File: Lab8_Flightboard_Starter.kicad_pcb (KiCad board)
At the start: 2 copper layers, 80 x 80 mm, 64 parts, among them J1 Motor1, J10 ESC3_GND, J11 ESC4_VBAT, J12 ESC4_GND, J2 Motor2, J3 Motor3, J4 Motor4, J5 ESC1_VBAT, J6 ESC1_GND, J7 ESC2_VBAT, J8 ESC2_GND, J9 ESC3_VBAT, Q1 DMP6023LE-13, U1 Teensy4.0, U2 TPS62933, U4 LP5912-3.3DRV, U5 LP5912-3.3DRV, U6 NRF24L01_Breakout, U9 LSM6DSO32_Adafruit

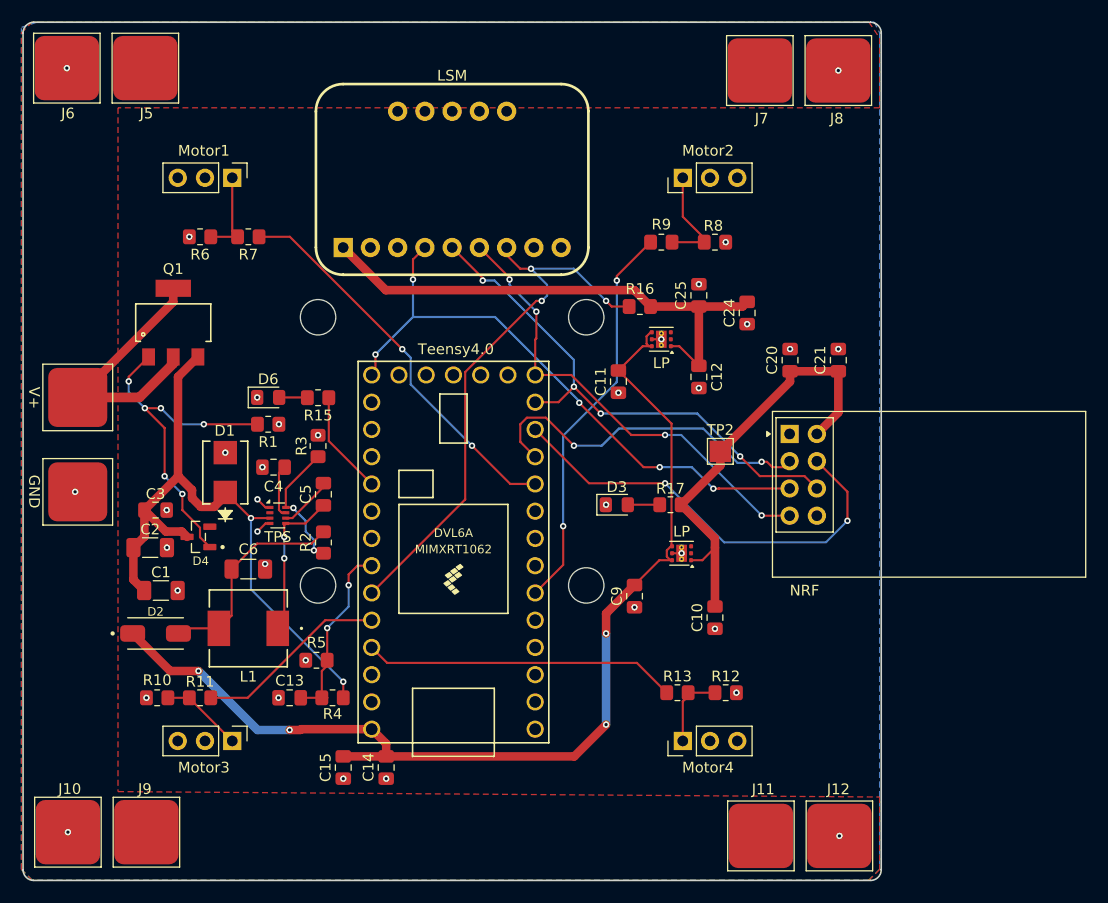
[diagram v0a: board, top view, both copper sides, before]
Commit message: Edited some dimensions
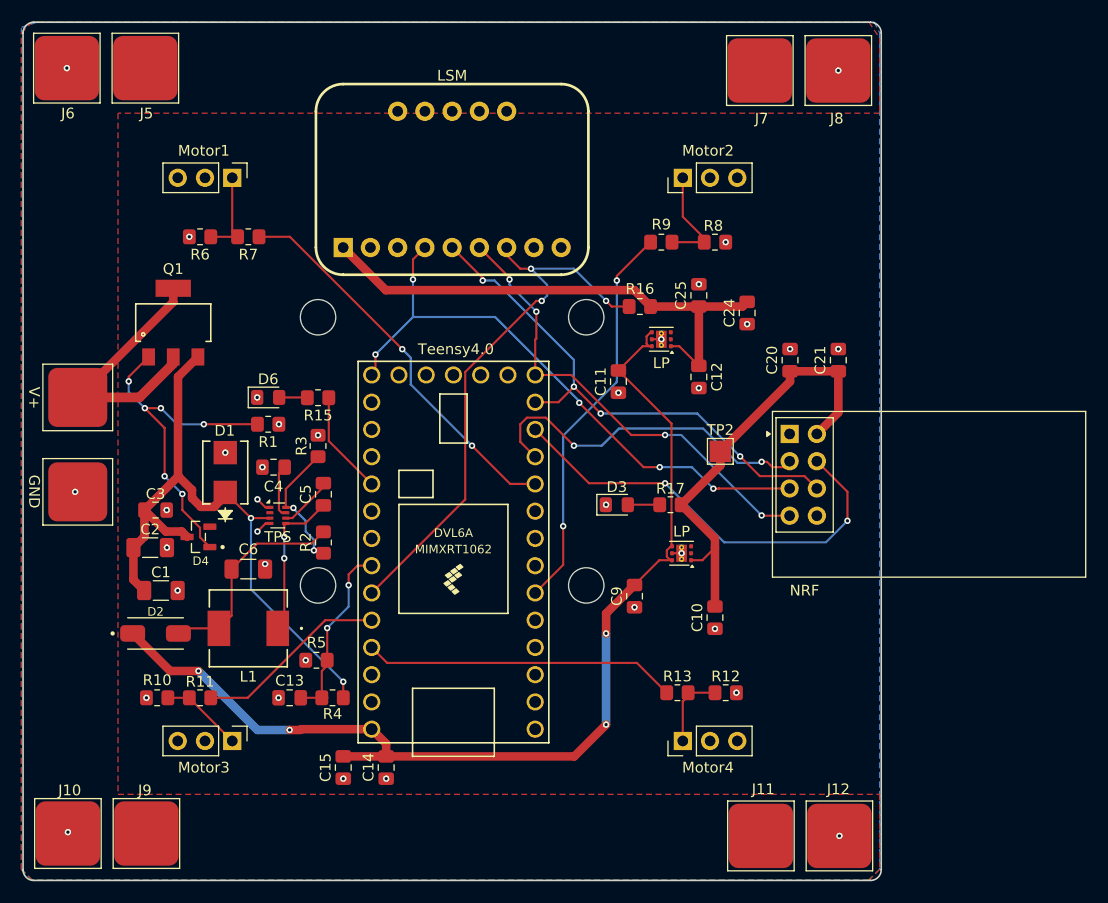
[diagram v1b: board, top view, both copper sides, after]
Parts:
- moved J10 0.12 mm to (111.4, 134.0)
- moved J9 0.12 mm to (118.8, 134.0)
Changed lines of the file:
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@@
 	(footprint "FC_Mechanical:Pad_x1_6mm"
 		(layer "F.Cu")
-		(at 111.431698 133.875 180)
+		(at 111.431698 134 180)
 		(property "Reference" "J10"
 			(at -0.068302 3.875 0)
@@
 			(polygon
 				(pts
-					(xy 114.431698 137.278308) (xy 108.231698 137.278308) (xy 108.231698 130.77169) (xy 114.431698 130.77169)
+					(xy 114.431698 137.403308) (xy 108.231698 137.403308) (xy 108.231698 130.89669) (xy 114.431698 130.89669)
 				)
 			)
@@
 	(footprint "FC_Mechanical:Pad_x1_6mm"
 		(layer "F.Cu")
-		(at 118.75 133.875 180)
+		(at 118.75 134 180)
 		(property "Reference" "J9"
 			(at 0.25 3.875 0)
@@
 			(polygon
 				(pts
-					(xy 121.75 137.278308) (xy 115.55 137.278308) (xy 115.55 130.77169) (xy 121.75 130.77169)
+					(xy 121.75 137.403308) (xy 115.55 137.403308) (xy 115.55 130.89669) (xy 121.75 130.89669)
 				)
 			)
@@
 	)
 	(segment
-		(start 116.5 131.875)
-		(end 118.65 134.025)
+		(start 126.989 103.3432)
+		(end 126 102.3542)
+		(width 0.2)
+		(layer "F.Cu")
+		(net "/SYS_VIN")
+	)
+	(segment
+		(start 117.4375 107.5)
+		(end 117.4375 110.5)
 		(width 0.8)
 		(layer "F.Cu")
-		(net "/VBAT")
+		(net "/SYS_VIN")
 	)
 	(segment
-		(start 118 93.5)
-		(end 112.25 93.5)
-		(width 0.9)
+		(start 118.4625 106.475)
+		(end 117.4375 107.5)
+		(width 0.8)
 		(layer "F.Cu")
-		(net "/VBAT")
+		(net "/SYS_VIN")
 	)
 	(segment
-		(start 121.15 83.325)
-		(end 121.15 84.6)
+		(start 124.965886 103.7)
+		(end 123.727207 103.7)
 		(width 0.8)
 		(layer "F.Cu")
-		(net "/VBAT")
+		(net "/SYS_VIN")
 	)
 	(segment
-		(start 121.15 89.725)
-		(end 121.15 90.35)
-		(width 0.9)
+		(start 128.3958 104.75)
+		(end 126 102.3542)
+		(width 0.2)
 		(layer "F.Cu")
-		(net "/VBAT")
+		(net "/SYS_VIN")
 	)
 	(segment
-		(start 121.15 84.6)
-		(end 112.25 93.5)
+		(start 118.4625 104)
+		(end 118.4625 106.475)
 		(width 0.8)
 		(layer "F.Cu")
-		(net "/VBAT")
+		(net "/SYS_VIN")
 	)
 	(segment
-		(start 121.15 90.35)
-		(end 118 93.5)
-		(width 0.9)
+		(start 130.16 104.75)
+		(end 128.3958 104.75)
+		(width 0.2)
 		(layer "F.Cu")
-		(net "/VBAT")
+		(net "/SYS_VIN")
+	)
+	(segment
+		(start 118.4625 104)
+		(end 120.4625 106)
+		(width 0.8)
+		(layer "F.Cu")
+		(net "/SYS_VIN")
+	)
+	(segment
+		(start 137 121.5)
+		(end 137 120)
+		(width 0.2)
+		(layer "F.Cu")
+		(net "/SYS_VIN")
+	)
+	(segment
+		(start 123.45 89.725)
+		(end 121.595 91.58)
+		(width 0.8)
+		(layer "F.Cu")
+		(net "/SYS_VIN")
+	)
+	(segment
+		(start 117.4375 110.5)
+		(end 118.4375 111.5)
+		(width 0.8)
+		(layer "F.Cu")
+		(net "/SYS_VIN")
+	)
+	(segment
+		(start 126 102.3542)
+		(end 126 102.665886)
+		(width 0.8)
+		(layer "F.Cu")
+		(net "/SYS_VIN")
+	)
+	(segment
+		(start 123.727207 103.7)
+		(end 122.9 102.872793)
+		(width 0.8)
+		(layer "F.Cu")
+		(net "/SYS_VIN")
+	)
+	(segment
+		(start 126 102.665886)
+		(end 124.965886 103.7)
+		(width 0.8)
+		(layer "F.Cu")
+		(net "/SYS_VIN")
+	)
+	(segment
+		(start 122.9 102.127207)
+		(end 121.640293 100.8675)
+		(width 0.8)
+		(layer "F.Cu")
+		(net "/SYS_VIN")
+	)
+	(segment
+		(start 120.4625 106)
+		(end 121.94 106)
+		(width 0.8)
+		(layer "F.Cu")
+		(net "/SYS_VIN")
+	)
+	(segment
+		(start 121.94 106)
+		(end 122.44 106.5)
+		(width 0.8)
+		(layer "F.Cu")
+		(net "/SYS_VIN")
+	)
+	(segment
+		(start 121.595 91.58)
+		(end 121.595 100.8675)
+		(width 0.8)
+		(layer "F.Cu")
+		(net "/SYS_VIN")
+	)
+	(segment
+		(start 121.640293 100.8675)
+		(end 121.595 100.8675)
+		(width 0.8)
+		(layer "F.Cu")
+		(net "/SYS_VIN")
+	)
+	(segment
+		(start 122.9 102.872793)
+		(end 122.9 102.127207)
+		(width 0.8)
+		(layer "F.Cu")
+		(net "/SYS_VIN")
+	)
+	(segment
+		(start 121.595 100.8675)
+		(end 118.4625 104)
+		(width 0.8)
+		(layer "F.Cu")
+		(net "/SYS_VIN")
+	)
+	(via
+		(at 128.3958 104.75)
+		(size 0.6)
+		(drill 0.3)
+		(layers "F.Cu" "B.Cu")
+		(net "/SYS_VIN")
+	)
+	(via
+		(at 137 120)
+		(size 0.6)
+		(drill 0.3)
+		(layers "F.Cu" "B.Cu")
+		(net "/SYS_VIN")
+	)
+	(segment
+		(start 128.3958 111.3958)
+		(end 128.3958 104.75)
+		(width 0.2)
+		(layer "B.Cu")
+		(net "/SYS_VIN")
+	)
+	(segment
+		(start 137 120)
+		(end 128.3958 111.3958)
+		(width 0.2)
+		(layer "B.Cu")
+		(net "/SYS_VIN")
 	)
 	(segment
@@
 	)
 	(segment
-		(start 126.989 103.3432)
-		(end 126 102.3542)
-		(width 0.2)
-		(layer "F.Cu")
-		(net "/SYS_VIN")
-	)
-	(segment
-		(start 117.4375 107.5)
-		(end 117.4375 110.5)
-		(width 0.8)
-		(layer "F.Cu")
-		(net "/SYS_VIN")
-	)
-	(segment
-		(start 118.4625 106.475)
-		(end 117.4375 107.5)
-		(width 0.8)
-		(layer "F.Cu")
-		(net "/SYS_VIN")
-	)
-	(segment
-		(start 124.965886 103.7)
-		(end 123.727207 103.7)
-		(width 0.8)
-		(layer "F.Cu")
-		(net "/SYS_VIN")
-	)
-	(segment
-		(start 128.3958 104.75)
-		(end 126 102.3542)
-		(width 0.2)
-		(layer "F.Cu")
-		(net "/SYS_VIN")
-	)
-	(segment
-		(start 118.4625 104)
-		(end 118.4625 106.475)
-		(width 0.8)
-		(layer "F.Cu")
-		(net "/SYS_VIN")
-	)
-	(segment
-		(start 130.16 104.75)
-		(end 128.3958 104.75)
-		(width 0.2)
-		(layer "F.Cu")
-		(net "/SYS_VIN")
-	)
-	(segment
-		(start 118.4625 104)
-		(end 120.4625 106)
-		(width 0.8)
-		(layer "F.Cu")
-		(net "/SYS_VIN")
-	)
-	(segment
-		(start 137 121.5)
-		(end 137 120)
-		(width 0.2)
-		(layer "F.Cu")
-		(net "/SYS_VIN")
-	)
-	(segment
-		(start 123.45 89.725)
-		(end 121.595 91.58)
-		(width 0.8)
-		(layer "F.Cu")
-		(net "/SYS_VIN")
-	)
-	(segment
-		(start 117.4375 110.5)
-		(end 118.4375 111.5)
-		(width 0.8)
-		(layer "F.Cu")
-		(net "/SYS_VIN")
-	)
-	(segment
-		(start 126 102.3542)
-		(end 126 102.665886)
-		(width 0.8)
-		(layer "F.Cu")
-		(net "/SYS_VIN")
-	)
-	(segment
-		(start 123.727207 103.7)
-		(end 122.9 102.872793)
-		(width 0.8)
-		(layer "F.Cu")
-		(net "/SYS_VIN")
-	)
-	(segment
-		(start 126 102.665886)
-		(end 124.965886 103.7)
-		(width 0.8)
-		(layer "F.Cu")
-		(net "/SYS_VIN")
-	)
-	(segment
-		(start 122.9 102.127207)
-		(end 121.640293 100.8675)
-		(width 0.8)
-		(layer "F.Cu")
-		(net "/SYS_VIN")
-	)
-	(segment
-		(start 120.4625 106)
-		(end 121.94 106)
-		(width 0.8)
-		(layer "F.Cu")
-		(net "/SYS_VIN")
-	)
-	(segment
-		(start 121.94 106)
-		(end 122.44 106.5)
-		(width 0.8)
-		(layer "F.Cu")
-		(net "/SYS_VIN")
-	)
-	(segment
-		(start 121.595 91.58)
-		(end 121.595 100.8675)
-		(width 0.8)
-		(layer "F.Cu")
-		(net "/SYS_VIN")
-	)
-	(segment
-		(start 121.640293 100.8675)
-		(end 121.595 100.8675)
-		(width 0.8)
-		(layer "F.Cu")
-		(net "/SYS_VIN")
-	)
-	(segment
-		(start 122.9 102.872793)
-		(end 122.9 102.127207)
-		(width 0.8)
-		(layer "F.Cu")
-		(net "/SYS_VIN")
-	)
-	(segment
-		(start 121.595 100.8675)
-		(end 118.4625 104)
-		(width 0.8)
-		(layer "F.Cu")
-		(net "/SYS_VIN")
-	)
-	(via
-		(at 128.3958 104.75)
-		(size 0.6)
-		(drill 0.3)
-		(layers "F.Cu" "B.Cu")
-		(net "/SYS_VIN")
-	)
-	(via
-		(at 137 120)
-		(size 0.6)
-		(drill 0.3)
-		(layers "F.Cu" "B.Cu")
-		(net "/SYS_VIN")
-	)
-	(segment
-		(start 128.3958 111.3958)
-		(end 128.3958 104.75)
-		(width 0.2)
-		(layer "B.Cu")
-		(net "/SYS_VIN")
-	)
-	(segment
-		(start 137 120)
-		(end 128.3958 111.3958)
-		(width 0.2)
-		(layer "B.Cu")
-		(net "/SYS_VIN")
-	)
-	(segment
 		(start 168.65 76.65)
 		(end 168.65 73.025)
@@
 	)
 	(segment
+		(start 116.5 131.875)
+		(end 118.65 134.025)
+		(width 0.8)
+		(layer "F.Cu")
+		(net "/VBAT")
+	)
+	(segment
+		(start 118 93.5)
+		(end 112.25 93.5)
+		(width 0.9)
+		(layer "F.Cu")
+		(net "/VBAT")
+	)
+	(segment
+		(start 121.15 83.325)
+		(end 121.15 84.6)
+		(width 0.8)
+		(layer "F.Cu")
+		(net "/VBAT")
+	)
+	(segment
+		(start 121.15 89.725)
+		(end 121.15 90.35)
+		(width 0.9)
+		(layer "F.Cu")
+		(net "/VBAT")
+	)
+	(segment
+		(start 121.15 84.6)
+		(end 112.25 93.5)
+		(width 0.8)
+		(layer "F.Cu")
+		(net "/VBAT")
+	)
+	(segment
+		(start 121.15 90.35)
+		(end 118 93.5)
+		(width 0.9)
+		(layer "F.Cu")
+		(net "/VBAT")
+	)
+	(segment
 		(start 122 104)
 		(end 122 102.5)
@@
 		(polygon
 			(pts
-				(xy 107 59.5) (xy 108 58.5) (xy 186 58.5) (xy 187 60) (xy 187 66.5) (xy 116 66.5) (xy 116 130.24468)
-				(xy 187 130.748226) (xy 187 137.5) (xy 186 138.5) (xy 108 138.5) (xy 107 137.5)
+				(xy 107 59.5) (xy 108 58.5) (xy 186 58.5) (xy 187 60) (xy 187 67) (xy 116 67) (xy 116 130.5) (xy 187 130.5)
+				(xy 187 137.5) (xy 186 138.5) (xy 108 138.5) (xy 107 137.5)
 			)
 		)
